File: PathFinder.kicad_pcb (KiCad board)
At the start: 2 copper layers, 65 x 77.5 mm, 13 parts, among them SW1 SW_Push, SW2 SW_Push, SW3 SW_Push, SW4 SW_Push, SW5 SW_Push, SW6 SW_Push, U1 XIAO-RP2040-DIP

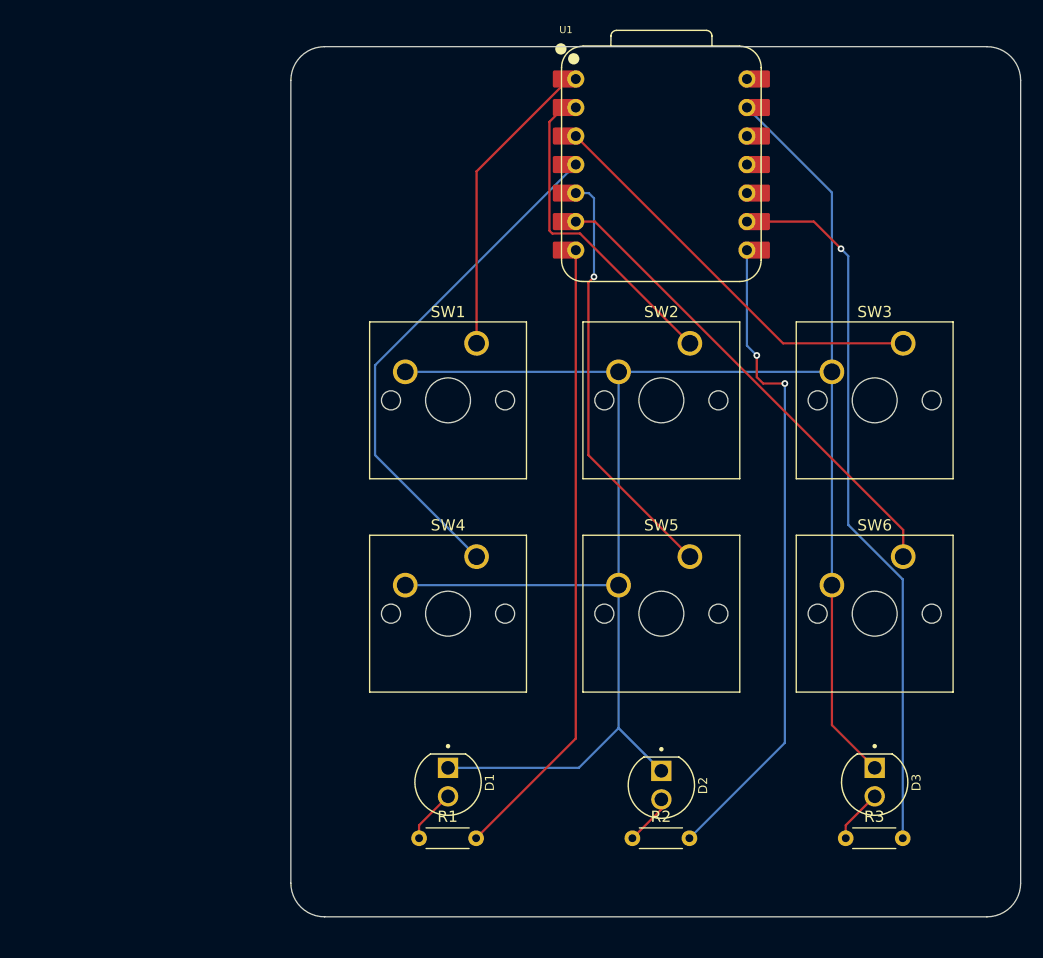
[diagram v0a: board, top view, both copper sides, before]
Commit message: Add files via upload
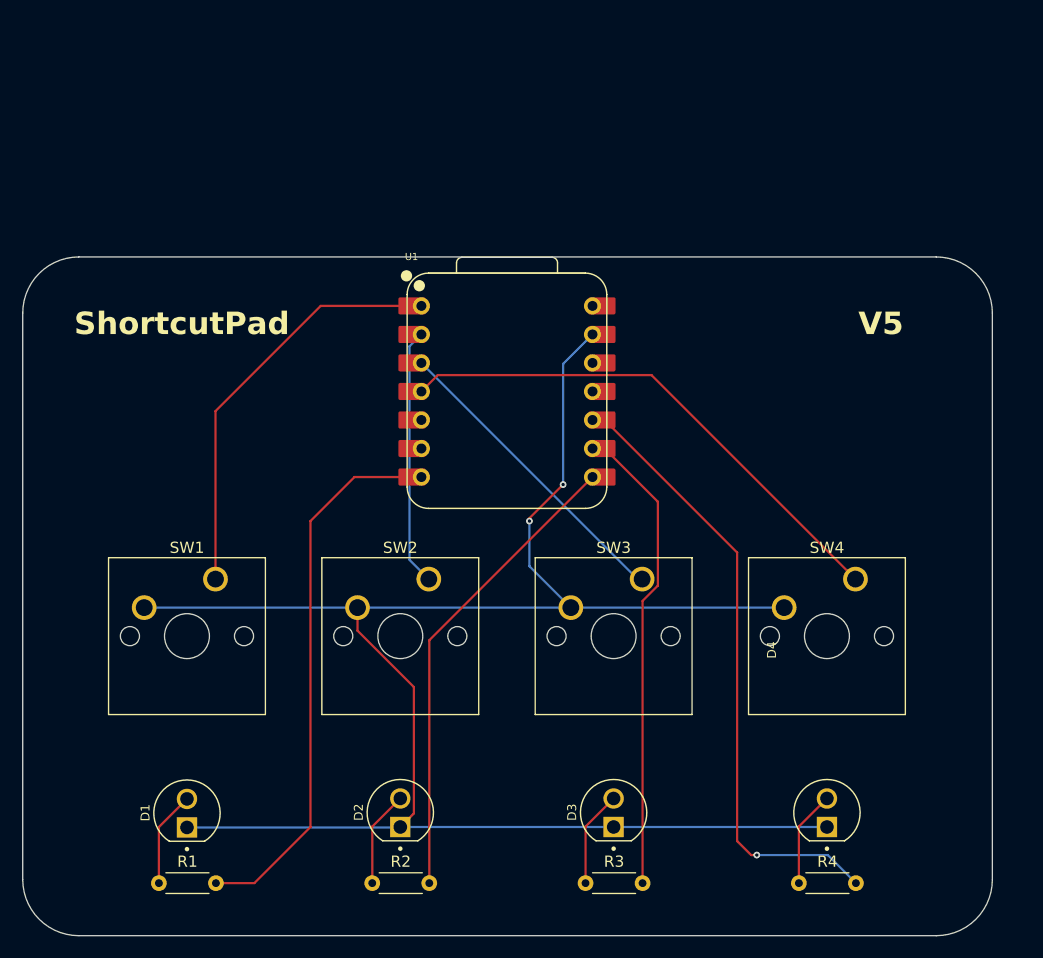
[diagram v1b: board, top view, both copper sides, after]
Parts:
- removed SW5, SW6: SW_Push, Button_Switch_Keyboard:SW_Cherry_MX_1.00u_PCB
- added D4: L08R5000Q1, footprints:LEDRD254W57D500H1070, F.Cu at (142.7, 95.7)
- added R4: R, Resistor_THT:R_Axial_DIN0204_L3.6mm_D1.6mm_P5.08mm_Horizontal, F.Cu at (140.2, 102.0)
- moved SW4 33.8 mm to (145.3, 74.9)
- moved SW1 31.3 mm to (88.3, 74.9)
- moved SW2 31.3 mm to (107.3, 74.9)
- moved SW3 31.3 mm to (126.3, 74.9)
- moved U1 24.4 mm to (114.2, 58.2)
- moved R1 23.5 mm to (83.2, 102.0)
- moved R2 23.5 mm to (102.2, 102.0)
- moved R3 23.5 mm to (121.2, 102.0)
- moved D1 23.4 mm to (85.7, 95.8), turned to 90 degrees
- moved D3 23.4 mm to (123.7, 95.7), turned to 90 degrees
- moved D2 23.4 mm to (104.7, 95.7), turned to 90 degrees
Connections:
- U1 pad 10: unconnected-(U1-GPIO4/MISO-Pad10) -> LED4
- U1 pad 5: button5 -> unconnected-(U1-GPIO6/SDA-Pad5)
- U1 pad 6: button6 -> unconnected-(U1-GPIO7/SCL-Pad6)
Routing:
- net LED4: track 0.00 -> 55.6 mm, vias 0 -> 1
- net button6: track 42.9 -> 0.00 mm
- net button5: track 37.7 -> 0.00 mm, vias 1 -> 0
- net LED3: track 64.2 -> 42.3 mm, vias 1 -> 0
- net LED2: track 58.4 -> 42.2 mm, vias 2 -> 0
- net GND: track 174.3 -> 164.3 mm, vias 0 -> 2
- net button1: track 27.6 -> 37.2 mm
- net button3: track 36.8 -> 27.6 mm
- net Net-(D4-PadA): track 0.00 -> 8.58 mm
- net LED1: track 56.1 -> 49.2 mm
- net button2: track 29.2 -> 22.9 mm
- net Net-(D2-PadA): track 4.53 -> 8.58 mm
- net Net-(D3-PadA): track 4.80 -> 8.58 mm
- net Net-(D1-PadA): track 4.80 -> 8.54 mm
- net button4: track 46.1 -> 46.8 mm
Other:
- board size 65 x 77.5 mm -> 86.4 x 60.5 mm
- board text added: "ShortcutPad"
- board text added: "V5"
